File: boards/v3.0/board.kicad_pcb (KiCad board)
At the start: 2 copper layers, 115.2 x 103.9 mm, 66 parts, among them J1 KF301-2P, J2 KF301-2P, J3 KF301-2P, J4 KF301-2P, J5 KF301-2P, J6 KF301-2P, P1 Pin Header, P2 Pin Header, P3 Pin Header, P4 Pin Header, P5 Pin Header, SW1 SS-12D00G 4mm, SW2 SS-12D00G 4mm, T1 ZMPT101B, T2 ZMPT101B, T3 ZMPT101B, U1 TL082, U2 TL082, U3 TL082, U4 TL082, U5 TL082, U6 TL082

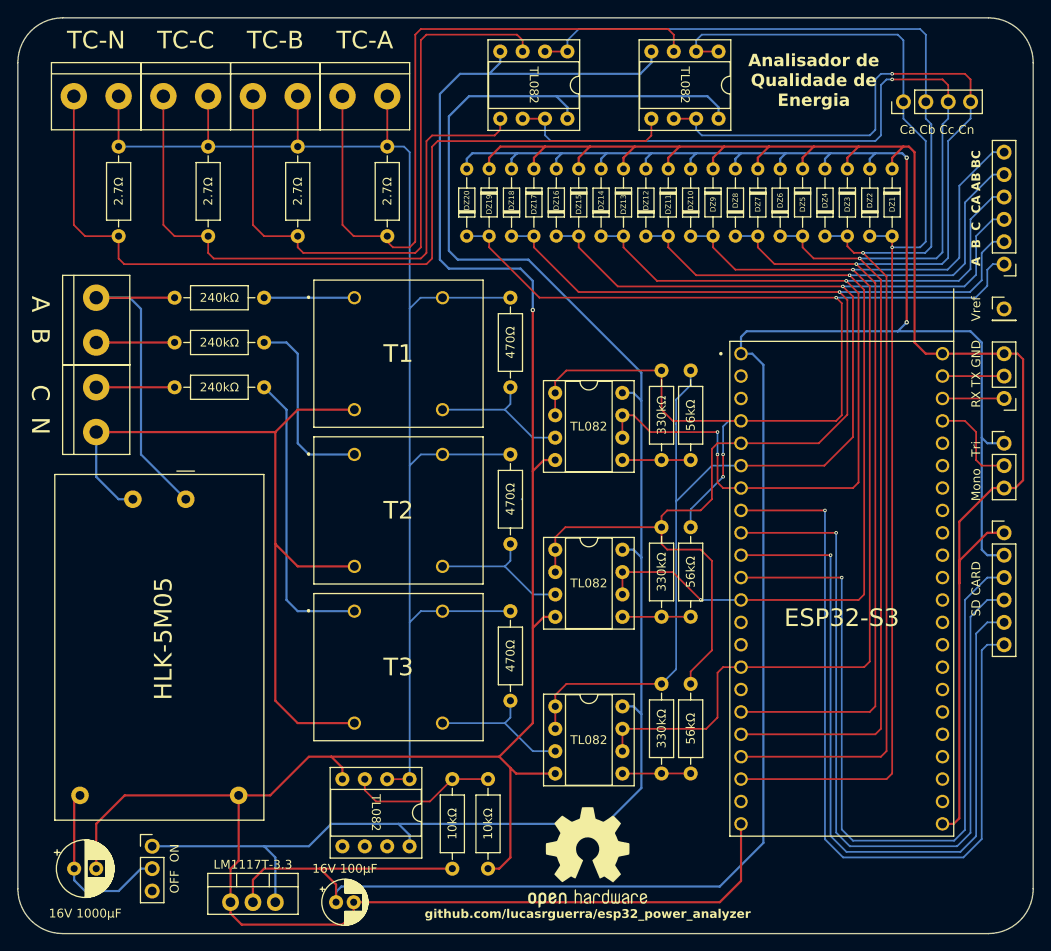
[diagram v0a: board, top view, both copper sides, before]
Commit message: Revision in the v3.0 board
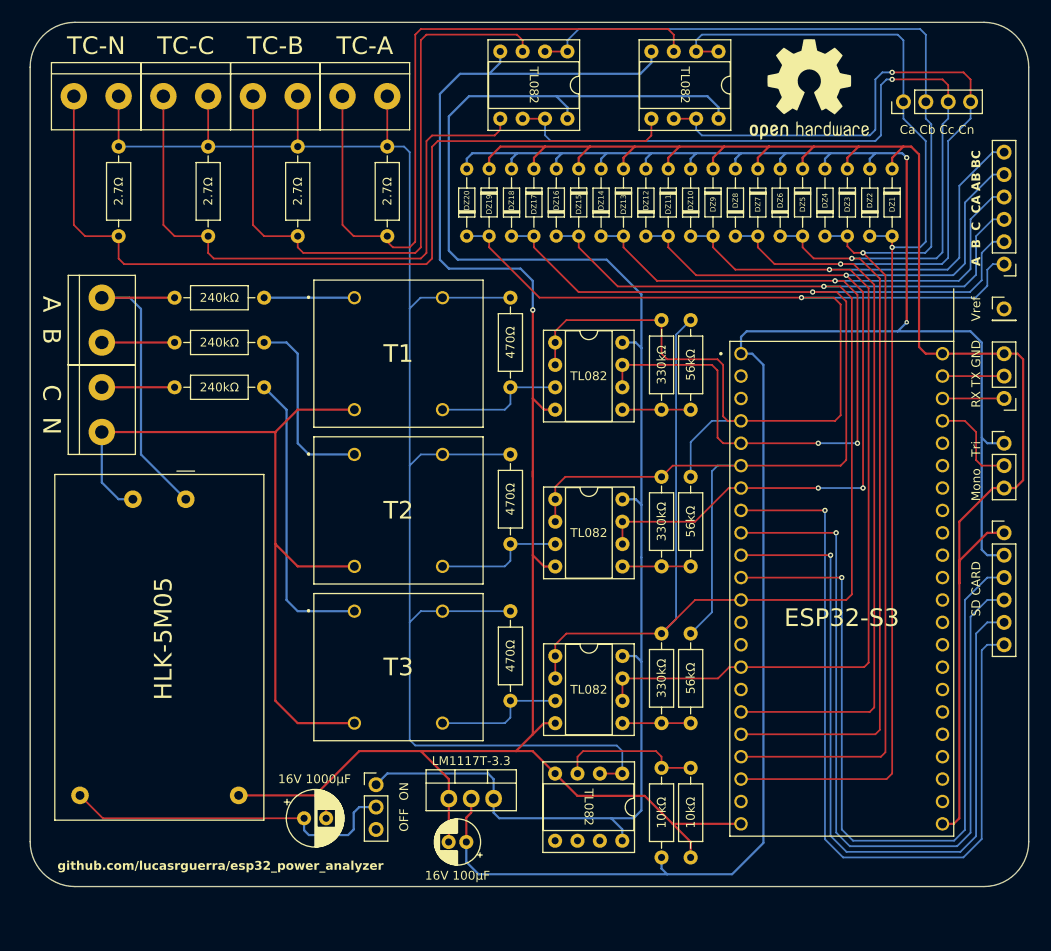
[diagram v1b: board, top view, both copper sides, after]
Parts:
- moved G*** 90.7 mm to (180.6, 43.7)
- moved PS2 27.4 mm to (139.7, 124.1)
- moved C1 26.7 mm to (123.3, 126.4)
- moved SW1 26.3 mm to (131.4, 122.6)
- moved U1 24.1 mm to (159.4, 121.3)
- moved R1 23.8 mm to (163.8, 130.8)
- moved R2 23.0 mm to (167.1, 120.7)
- moved C2 16.3 mm to (141.7, 129.1), turned to 180 degrees
- moved R10 5.72 mm to (167.1, 69.8)
- moved R11 5.72 mm to (163.8, 87.6)
- moved R12 5.72 mm to (167.1, 87.6)
- moved R13 5.72 mm to (163.8, 105.4)
- moved R14 5.72 mm to (167.1, 105.4)
- moved R9 5.72 mm to (163.8, 69.8)
- moved U2 5.72 mm to (151.8, 72.4)
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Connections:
- MCU1 pad J1_12: Treated Wave AB -> Treated Wave C
- MCU1 pad J1_5: Treated Wave B -> Treated Wave CA
- MCU1 pad J1_6: Treated Wave C -> Treated Wave B
- MCU1 pad J1_7: Treated Wave CA -> Treated Wave AB
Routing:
- net GND: track 460.3 -> 385.7 mm
- net Vcc: track 288.7 -> 251.8 mm
- net TC A-2: track 165.7 -> 188.4 mm
- net Vin: track 202.1 -> 179.7 mm
- net Treated Wave C: track 153.6 -> 173.7 mm
- net Power: track 20.3 -> 38.7 mm
- net Treated Wave AB: track 120.4 -> 108.4 mm, vias 2 -> 3
- net Treated Wave A: track 138.2 -> 142.6 mm, vias 3 -> 1
- net Treated Wave BC: track 130.2 -> 127.2 mm
- net Treated Wave CA: track 115.6 -> 113.2 mm
- net Wave B: track 16.9 -> 15.0 mm
- net Wave A: track 16.9 -> 14.9 mm
- net Wave C: track 16.9 -> 15.0 mm
- net Current N: track 156.0 -> 157.7 mm
- net Treated Wave B: track 148.0 -> 146.9 mm
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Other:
- board size 115.2 x 103.9 mm -> 113.3 x 98 mm
- board text removed: "Analisador de Qualidade de Energia"
